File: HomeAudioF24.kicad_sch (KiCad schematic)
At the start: 40 parts, among them U1 LF356M, U2 LF356M, U3 LF356M, U4 LF356M, U5 LF356M, U6 LF356M, U7 LF356M, U8 LF356M, U9 LF356M

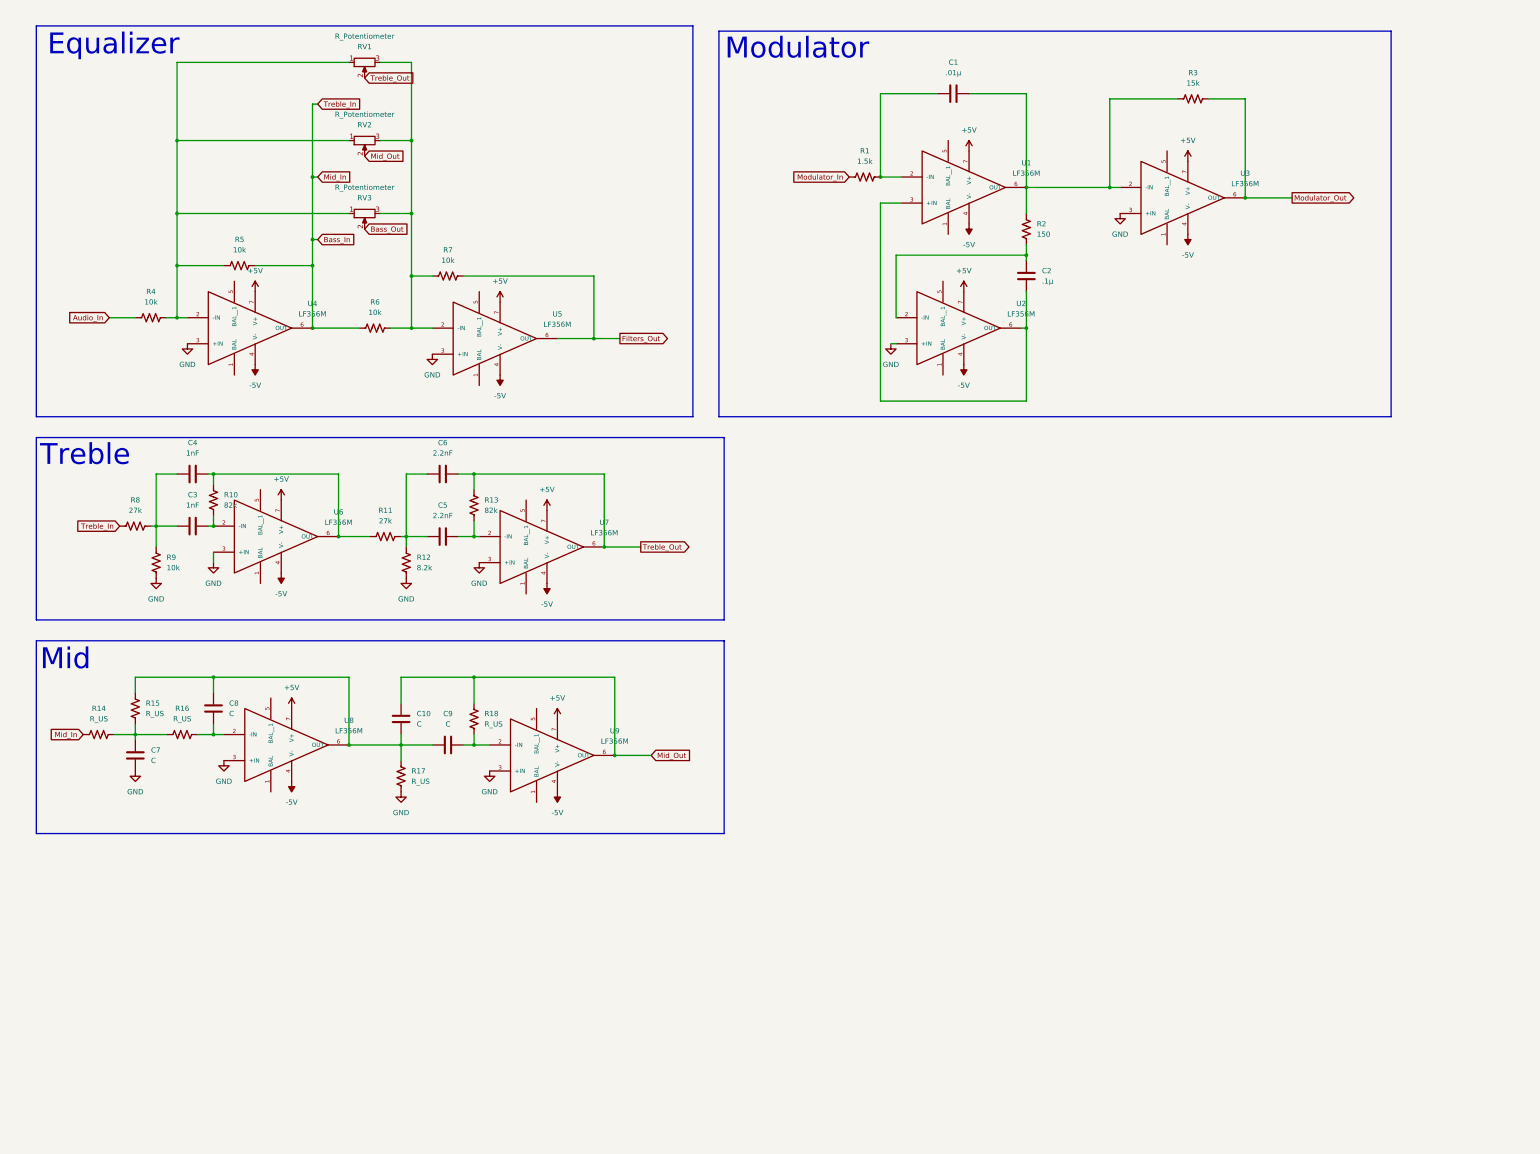
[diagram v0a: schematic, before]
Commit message: First Major Revision
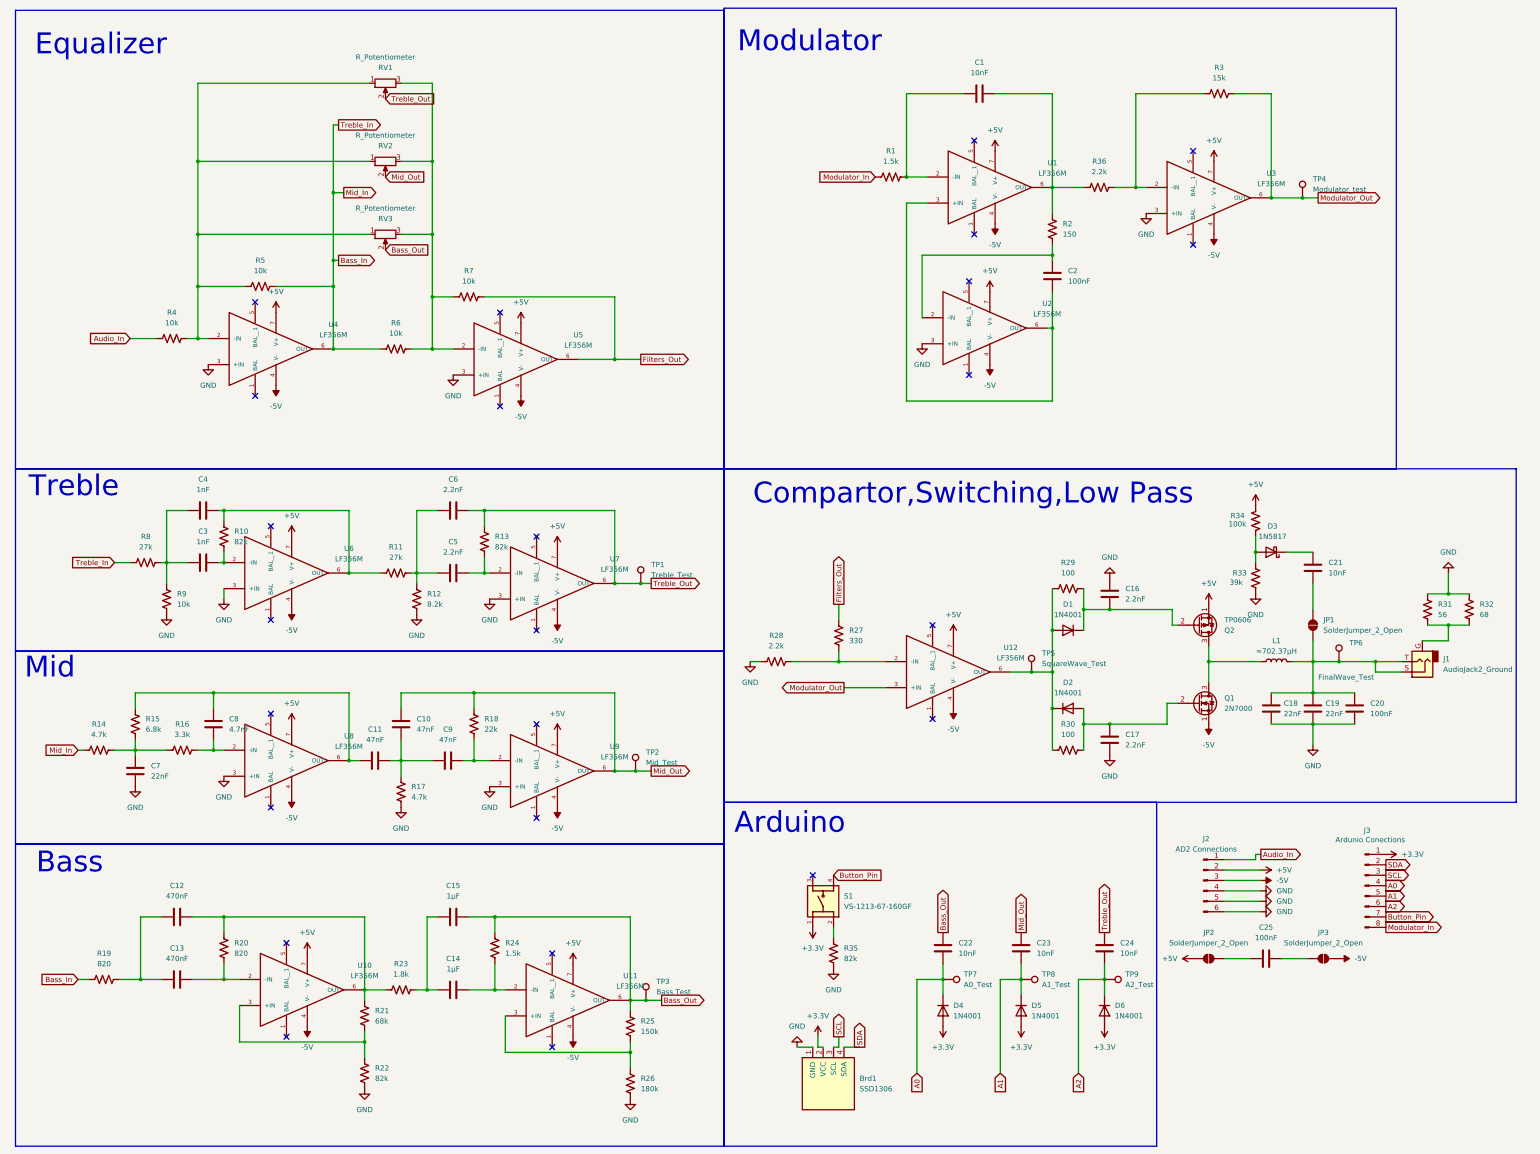
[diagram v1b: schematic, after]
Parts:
- added Brd1: SSD1306, Display_New:128x64OLED SSD1306, symbol SSD1306-128x64_OLED:SSD1306
- added C11: 47nF, ColorOrgan:C_Disc_D4.3mm_W1.9mm_P5.00mm_Handsolder, symbol Device:C
- added C12, C13: 470nF, ColorOrgan:R_Combo, symbol Device:C
- added C14, C15: 1μF, ColorOrgan:C_Disc_D4.3mm_W1.9mm_P5.00mm_Handsolder, symbol Device:C
- added C16, C17: 2.2nF, ColorOrgan:C_Disc_D4.3mm_W1.9mm_P5.00mm_Handsolder, symbol Device:C
- added C18, C19: 22nF, ColorOrgan:C_Disc_D4.3mm_W1.9mm_P5.00mm_Handsolder, symbol Device:C
- added C20, C25: 100nF, ColorOrgan:C_Disc_D4.3mm_W1.9mm_P5.00mm_Handsolder, symbol Device:C
- added C21, C22, C23, C24: 10nF, ColorOrgan:C_Disc_D4.3mm_W1.9mm_P5.00mm_Handsolder, symbol Device:C
- added D1, D2, D4, D5, D6: 1N4001, Diode_THT:D_DO-41_SOD81_P10.16mm_Horizontal, symbol Diode:1N4001
- added D3: 1N5817, Diode_THT:D_DO-41_SOD81_P10.16mm_Horizontal, symbol Diode:1N5817
- added J1: AudioJack2_Ground, ColorOrgan:Jack_3.5mm_Ground_RightAngle, symbol Connector_Audio:AudioJack2_Ground
- added J2: AD2 Connections, Connector_PinHeader_2.54mm:PinHeader_1x06_P2.54mm_Vertical, symbol Connector:Conn_01x06_Pin
- added J3: Ardunio Conections, Connector_PinHeader_2.54mm:PinHeader_1x08_P2.54mm_Vertical, symbol Connector:Conn_01x08_Pin
- added JP1, JP2, JP3: SolderJumper_2_Open, Jumper:SolderJumper-2_P1.3mm_Open_TrianglePad1.0x1.5mm, symbol Jumper:SolderJumper_2_Open
- added L1: ≈702.37μH, ColorOrgan:InductorCore, symbol Device:L
- added Q1: 2N7000, Package_TO_SOT_THT:TO-92_Inline, symbol Transistor_FET:2N7000
- added Q2: TP0606, Package_TO_SOT_THT:TO-92L_Inline, symbol Transistor_FET:TP0610L
- added R19, R20: 820, ColorOrgan:1_2W Res + 1206, symbol Device:R_US
- added R21: 68k, ColorOrgan:1_2W Res + 1206, symbol Device:R_US
- added R22, R35: 82k, ColorOrgan:1_2W Res + 1206, symbol Device:R_US
- added R23: 1.8k, ColorOrgan:1_2W Res + 1206, symbol Device:R_US
- added R24: 1.5k, ColorOrgan:1_2W Res + 1206, symbol Device:R_US
- added R25: 150k, ColorOrgan:1_2W Res + 1206, symbol Device:R_US
- added R26: 180k, ColorOrgan:1_2W Res + 1206, symbol Device:R_US
- added R27: 330, ColorOrgan:1_2W Res + 1206, symbol Device:R_US
- added R28, R36: 2.2k, ColorOrgan:1_2W Res + 1206, symbol Device:R_US
- added R29, R30: 100, ColorOrgan:1_2W Res + 1206, symbol Device:R_US
- added R31: 56, ColorOrgan:1_2W Res + 1206, symbol Device:R_US
- added R32: 68, ColorOrgan:1_2W Res + 1206, symbol Device:R_US
- added R33: 39k, ColorOrgan:1_2W Res + 1206, symbol Device:R_US
- added R34: 100k, ColorOrgan:1_2W Res + 1206, symbol Device:R_US
- added S1: VS-1213-67-160GF, 4PinButton:SW_VS-1213-67-160GF, symbol 4PinButton:VS-1213-67-160GF
- added TP1: Treble_Test, TestPoint:TestPoint_Pad_2.5x2.5mm, symbol Connector:TestPoint
- added TP2: Mid_Test, TestPoint:TestPoint_Pad_2.5x2.5mm, symbol Connector:TestPoint
- added TP3: Bass Test, TestPoint:TestPoint_Pad_2.5x2.5mm, symbol Connector:TestPoint
- added TP4: Modulator_test, TestPoint:TestPoint_Pad_2.5x2.5mm, symbol Connector:TestPoint
- added TP5: SquareWave_Test, TestPoint:TestPoint_Pad_2.5x2.5mm, symbol Connector:TestPoint
- added TP6: FinalWave_Test, TestPoint:TestPoint_Pad_2.5x2.5mm, symbol Connector:TestPoint
- added TP7: A0_Test, TestPoint:TestPoint_Pad_2.5x2.5mm, symbol Connector:TestPoint
- added TP8: A1_Test, TestPoint:TestPoint_Pad_2.5x2.5mm, symbol Connector:TestPoint
- added TP9: A2_Test, TestPoint:TestPoint_Pad_2.5x2.5mm, symbol Connector:TestPoint
- added U10, U11, U12: LF356M, Package_DIP:DIP-8_W7.62mm_LongPads, symbol LF356M:LF356M
- C1: value .01μ -> 10nF; footprint ColorOrgan:R_Combo -> ColorOrgan:C_Disc_D4.3mm_W1.9mm_P5.00mm_Handsolder
- C10, C9: value C -> 47nF; footprint (none) -> ColorOrgan:C_Disc_D4.3mm_W1.9mm_P5.00mm_Handsolder
- C2: value .1μ -> 100nF; footprint ColorOrgan:R_Combo -> ColorOrgan:C_Disc_D4.3mm_W1.9mm_P5.00mm_Handsolder
- C3, C4, C5, C6: footprint ColorOrgan:R_Combo -> ColorOrgan:C_Disc_D4.3mm_W1.9mm_P5.00mm_Handsolder
- C7: value C -> 22nF; footprint (none) -> ColorOrgan:C_Disc_D4.3mm_W1.9mm_P5.00mm_Handsolder
- C8: value C -> 4.7nF; footprint (none) -> ColorOrgan:C_Disc_D4.3mm_W1.9mm_P5.00mm_Handsolder
- R14, R17: value R_US -> 4.7k; footprint (none) -> ColorOrgan:1_2W Res + 1206
- R15: value R_US -> 6.8k; footprint (none) -> ColorOrgan:1_2W Res + 1206
- R16: value R_US -> 3.3k; footprint (none) -> ColorOrgan:1_2W Res + 1206
- R18: value R_US -> 22k; footprint (none) -> ColorOrgan:1_2W Res + 1206
- RV1, RV2, RV3: footprint (none) -> Potentiometer_THT:Potentiometer_Vishay_148-149_Single_Vertical
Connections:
- net +5V: now also J2.2 (Pin_2), JP2.2 (B), Q2.1 (S), R34.2, U10.7 (V+), U11.7 (V+), U12.7 (V+)
- net -5V: now also J2.3 (Pin_3), JP3.1 (A), Q1.1 (S), U10.4 (V-), U11.4 (V-), U12.4 (V-)
- net Audio_In: now also J2.1 (Pin_1)
- net Bass_In: now also R19.1
- net Bass_Out: now also C15.2, C22.1, R24.1, R25.1, TP3.1, U11.6 (OUT)
- net Filters_Out: now also R27.1
- net GND: now also Brd1.1 (GND), C16.1, C17.2, C18.1, C19.1, C20.1, J2.4 (Pin_4), J2.5 (Pin_5), J2.6 (Pin_6), R22.1, R26.2, R28.2, R31.1, R32.1, R33.2, R35.2
- net Mid_Out: now also C23.1, TP2.1
- net Modulator_In: now also J3.8 (Pin_8)
- net Modulator_Out: now also TP4.1, U12.3 (+IN)
- net Treble_Out: now also C24.1, TP1.1
- net at C10.2, C9.2, R17.1: now also C11.2; no longer C8.2, R15.2, U8.6 (OUT)
- net at C1.2, R2.2, U1.6 (OUT): now also R36.1; no longer R3.1, U3.2 (-IN)
- new net: C25.2, JP3.2 (B)
- new net: R35.1, S1.2
- new net: R27.2, R28.1, U12.2 (-IN)
- new net: C13.2, R20.1, U10.2 (-IN)
- new net: C12.2, R20.2, R21.2, R23.2, U10.6 (OUT)
- new net: D1.2 (A), D2.1 (K), R29.1, R30.1, TP5.1, U12.6 (OUT)
- new net: C17.1, D2.2 (A), Q1.2 (G), R30.2
- new net: C18.2, C19.2, C20.2, J1.S, J1.T, JP1.1 (A), L1.2, TP6.1
- new net: D3.2 (A), R33.1, R34.1
- new net: C12.1, C13.1, R19.2
- new net: L1.1, Q1.3 (D), Q2.3 (D)
- new net: R21.1, R22.2, U10.3 (+IN)
- new net: R3.1, R36.2, U3.2 (-IN)
- new net: C14.1, C15.1, R23.1
- new net: C21.1, D3.1 (K)
- new net: C21.2, JP1.2 (B)
- new net: C25.1, JP2.1 (A)
- new net: C11.1, C8.2, R15.2, U8.6 (OUT)
- new net: J1.G, R31.2, R32.2
- new net: C14.2, R24.2, U11.2 (-IN)
- new net: R25.2, R26.1, U11.3 (+IN)
- new net: C16.2, D1.1 (K), Q2.2 (G), R29.2
- new net +3.3V: Brd1.2 (VCC), D4.2 (A), D5.2 (A), D6.2 (A), J3.1 (Pin_1), S1.1
- new net A0: C22.2, D4.1 (K), J3.4 (Pin_4), TP7.1
- new net A1: C23.2, D5.1 (K), J3.5 (Pin_5), TP8.1
- new net A2: C24.2, D6.1 (K), J3.6 (Pin_6), TP9.1
- new net Button_Pin: J3.7 (Pin_7), S1.4
- new net SCL: Brd1.3 (SCL), J3.3 (Pin_3)
- new net SDA: Brd1.4 (SDA), J3.2 (Pin_2)
- no-connect marks 0 -> 25
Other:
- note added: "Arduino"
- note added: "Bass"
- note added: "Compartor,Switching,Low Pass"
- moved on the sheet: C1, C10, C2, C3, C4, C5, C6, C7, C8, C9, R1, R10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
